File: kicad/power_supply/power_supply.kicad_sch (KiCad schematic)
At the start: 54 parts, among them J1 Conn_WallSocket_Earth, J2 USB_C_Receptacle_USB2.0, J3 Conn_01x02, J4 Conn_02x08_Odd_Even, J5 Conn_WallSocket_Earth, Q1 BCM53DS, Q2 BCM56DS, SW1 SW_SPST, T1 70043K, U1 PCM2706CPJTR, Y1 12MHz±0.05%

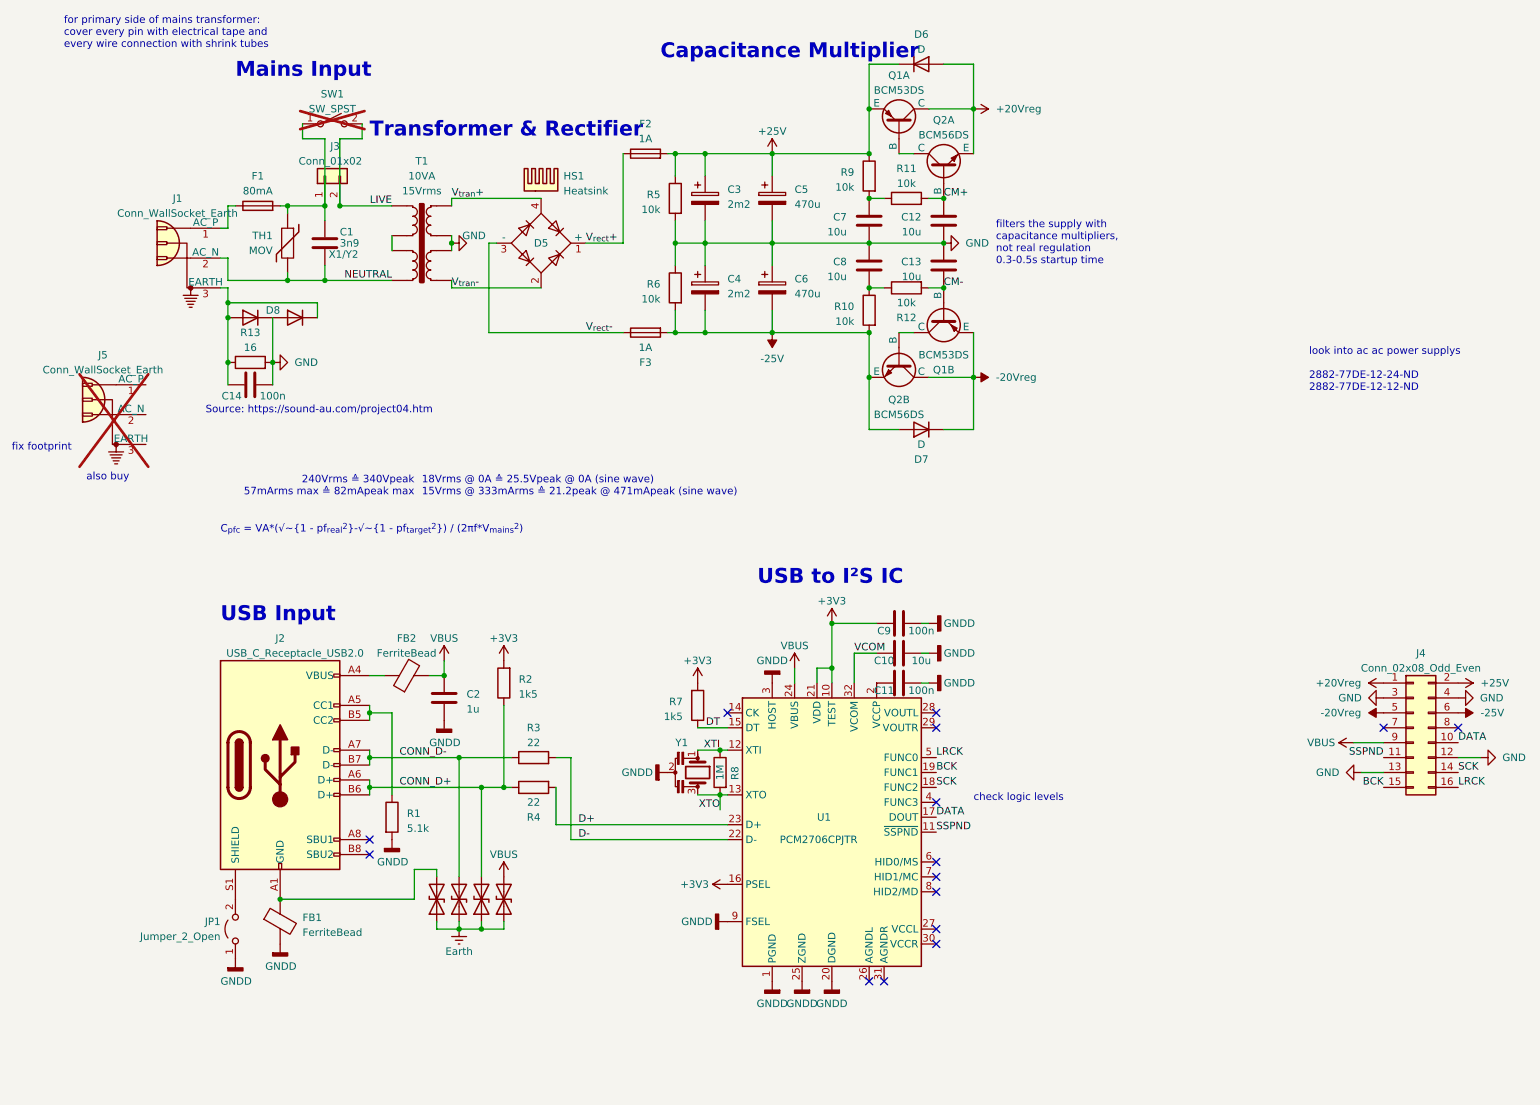
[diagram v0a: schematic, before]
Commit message: commit
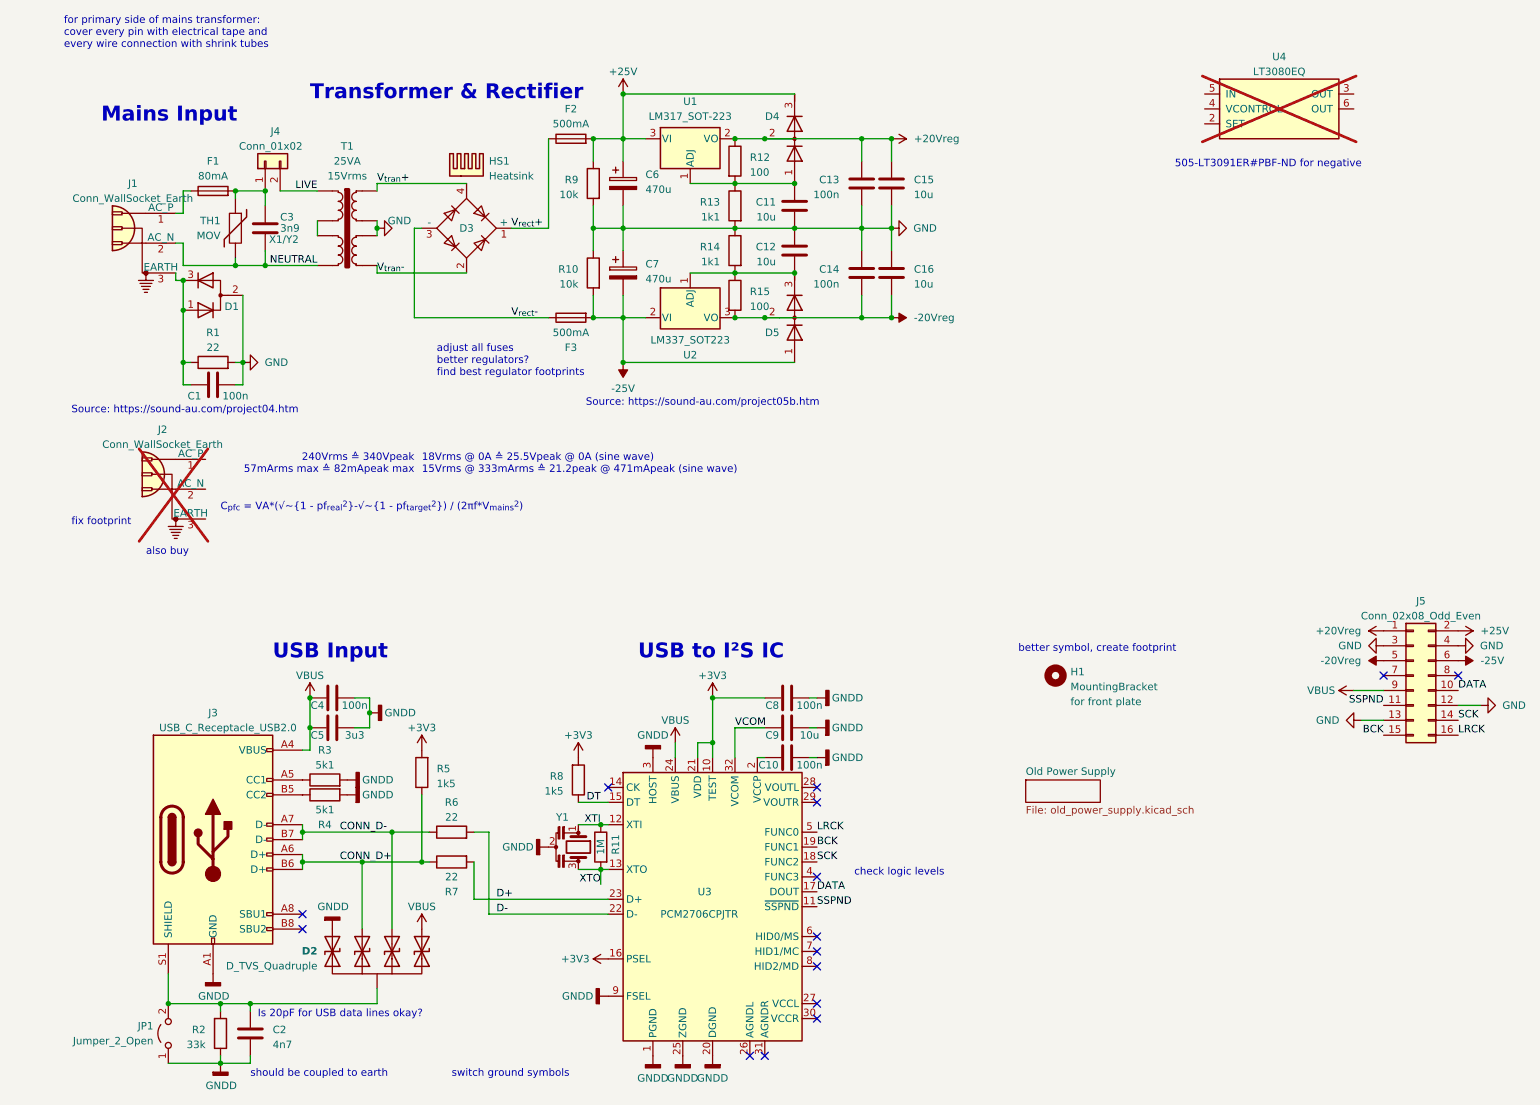
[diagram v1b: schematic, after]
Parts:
- removed C3, C4: 2m2, Capacitor_THT:CP_Radial_D12.5mm_P5.00mm, symbol Device:C_Polarized
- removed C5: 470u, Capacitor_THT:CP_Radial_D10.0mm_P5.00mm, symbol Device:C_Polarized
- removed C7, C8: 10u, Capacitor_SMD:C_1206_3216Metric_Pad1.33x1.80mm_HandSolder, symbol Device:C
- removed D1, D2, D3, D4: D_TVS, symbol Device:D_TVS
- removed D6, D7: D, Diode_SMD:D_SOD-323_HandSoldering, symbol Device:D
- removed D8: ~, Package_TO_SOT_SMD:SOT-23-3, symbol library:Dual_Diode_Array
- removed FB1, FB2: FerriteBead, symbol Device:FerriteBead
- removed Q1: BCM53DS, Package_SO:SC-74-6_1.5x2.9mm_P0.95mm, symbol library:Dual-PNP
- removed Q2: BCM56DS, Package_SO:SC-74-6_1.5x2.9mm_P0.95mm, symbol library:Dual-NPN
- removed R1: 5.1k, Resistor_SMD:R_1206_3216Metric_Pad1.30x1.75mm_HandSolder, symbol Device:R
- removed R10, R11, R9: 10k, Resistor_SMD:R_1206_3216Metric_Pad1.30x1.75mm_HandSolder, symbol Device:R
- removed SW1: SW_SPST, symbol Switch:SW_SPST
- added C11, C15, C16: 10u, Capacitor_SMD:C_1206_3216Metric_Pad1.33x1.80mm_HandSolder, symbol Device:C
- added C14, C4: 100n, Capacitor_SMD:C_1206_3216Metric_Pad1.33x1.80mm_HandSolder, symbol Device:C
- added C5: 3u3, Capacitor_SMD:C_1206_3216Metric_Pad1.33x1.80mm_HandSolder, symbol Device:C
- added C7: 470u, Capacitor_THT:CP_Radial_D10.0mm_P5.00mm, symbol Device:C_Polarized
- added D1: ~, Package_TO_SOT_SMD:SOT-23-3, symbol Device:D_Dual_Series_ACK_Parallel
- added D2: D_TVS_Quadruple, Package_TO_SOT_SMD:SOT-353_SC-70-5_Handsoldering, symbol library:D_TVS_Quadruple
- added D4, D5: ~, Package_TO_SOT_SMD:SOT-23-3, symbol Device:D_Dual_Series_ACK
- added H1: MountingBracket, symbol Mechanical:MountingHole
- added R13, R14: 1k1, Resistor_SMD:R_1206_3216Metric_Pad1.30x1.75mm_HandSolder, symbol Device:R
- added R15: 100, Resistor_SMD:R_1206_3216Metric_Pad1.30x1.75mm_HandSolder, symbol Device:R
- added R2: 33k, Resistor_SMD:R_1206_3216Metric_Pad1.30x1.75mm_HandSolder, symbol Device:R
- added R3, R4: 5k1, Resistor_SMD:R_1206_3216Metric_Pad1.30x1.75mm_HandSolder, symbol Device:R
- added U1: LM317_SOT-223, Package_TO_SOT_SMD:SOT-223-3_TabPin2, symbol Regulator_Linear:LM317_SOT-223
- added U2: LM337_SOT223, Package_TO_SOT_SMD:SOT-223-3_TabPin2, symbol Regulator_Linear:LM337_SOT223
- added U4: LT3080EQ, Package_TO_SOT_SMD:TO-263-5_TabPin3, symbol Regulator_Linear:LT3080xQ
- C13: value 10u -> 100n; Digikey 1276-3100-1-ND -> (none)
- C2: value 1u -> 4n7
- F2, F3: value 1A -> 500mA; footprint Fuse:Fuse_1206_3216Metric_Pad1.42x1.75mm_HandSolder -> Fuse:Fuse_Schurter_UMT250; Digikey 507-1891-1-ND -> 486-3478-1-ND
- R1: renamed from R13; value 16 -> 22
- R12: value 10k -> 100
- T1: value 70043K -> 70063K; footprint library:Talema_Transformer_2P2S_10VA -> library:Talema_Transformer_2P2S_25VA; Digikey 1295-1043-ND -> 1295-1023-ND; Leistung 10VA -> 25VA
- U3: renamed from U1; Digikey (none) -> 296-40481-1-ND
- renumbered C14 to C1, C11 to C10, C1 to C3, C9 to C8, C10 to C9, D5 to D3, J5 to J2, J2 to J3, J3 to J4, J4 to J5, R6 to R10, R8 to R11, R2 to R5, R3 to R6, R4 to R7, R7 to R8, R5 to R9
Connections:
- net CM+ is gone; now on net GND: C12.1
- net +20Vreg: now also C13.1, R12.1, C15.1, D4.2 (common), U1.2 (VO)
- net +25V: now also C6.1, D4.3 (K), U1.3 (VI)
- net -20Vreg: now also C14.2, C16.2, D5.2 (common), R15.2, U2.3 (VO)
- net -25V: now also C7.2, D5.1 (A), U2.2 (VI); no longer C6.2
- net CONN_D+: now also D2.4 (A3)
- net CONN_D-: now also D2.3 (A2)
- net GND: now also C13.2, C6.2, C11.2, C14.1, C15.2, C16.1, C7.1, D1.2 (A), R13.2, R14.1; no longer C12.2, C13.1, C6.1
- net GNDD: now also C2.2, J3.A1 (GND), J3.A12 (GND), J3.B1 (GND), J3.B12 (GND), C4.1, C5.1, D2.5 (A4), R2.1, R3.2, R4.2; no longer C2.1
- net VBUS: now also J3.A4 (VBUS), J3.A9 (VBUS), J3.B4 (VBUS), J3.B9 (VBUS), C4.2, C5.2, D2.1 (A1); no longer C2.2
- net at C1.2, J1.3 (EARTH), R1.1: now also D1.1 (K), D1.3 (K)
- net at J3.A5 (CC1): now also R3.1; no longer J3.B5 (CC2)
- net at J3.S1 (SHIELD), JP1.2 (B): now also C2.1, D2.2 (C), R2.2
- net CM-: no longer names the net of R12.2
- net CM-: now also C11.1, D4.1 (A), R13.1, U1.1 (ADJ); no longer C13.2
- new net: C12.2, D5.3 (K), R14.2, R15.1, U2.1 (ADJ)
- new net: J3.B5 (CC2), R4.1
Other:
- added sheet Old Power Supply (old_power_supply.kicad_sch)
- note added: "505-LT3091ER#PBF-ND for negative"
- note added: "Is 20pF for USB data lines okay?"
- note added: "Source: https://sound-au.com/project05b.htm"
- note added: "adjust all fuses better regulators? find best regulator footprints"
- note added: "better symbol, create footprint"
- note added: "should be coupled to earth"
- note added: "switch ground symbols"
- note removed: "Capacitance Multiplier"
- note removed: "filters the supply with capacitance multipliers, not real regulation 0.3-0.5s startup time"
- note removed: "look into ac ac power supplys 2882-77DE-12-24-ND 2882-77DE-12-12-ND"
- moved on the sheet: C1, C10, C3, C8, C9, D3, F1, F2, HS1, J1, J2, J3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
